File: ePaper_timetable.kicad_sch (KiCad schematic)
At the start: 44 parts, among them J1 26 pin FPC connector 0.5 mm p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, J2 Charging input - 5V, J3 Jumpers, J4 Jumpers, J5 Battery connector, Q1 NMOS, Q2 FS8205A, Q3 PMOS, SW1 SW_Push, SW2 SW_Push, SW3 SW_Push, U1 TP4056, U2 DW01A

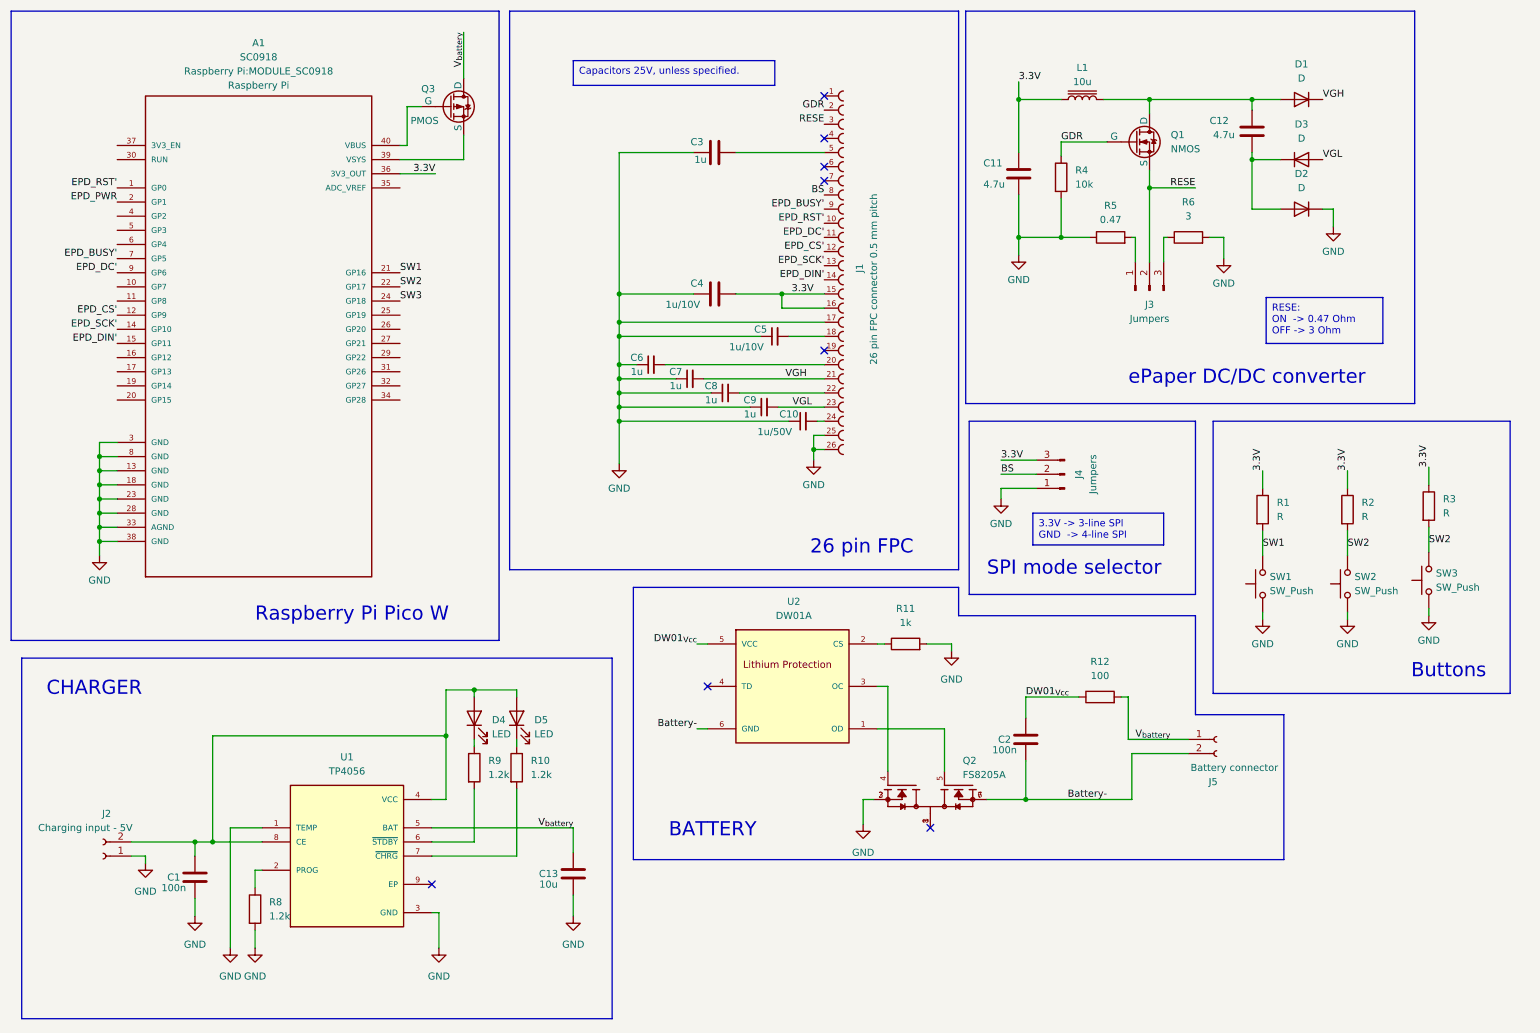
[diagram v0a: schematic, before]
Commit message: reference board
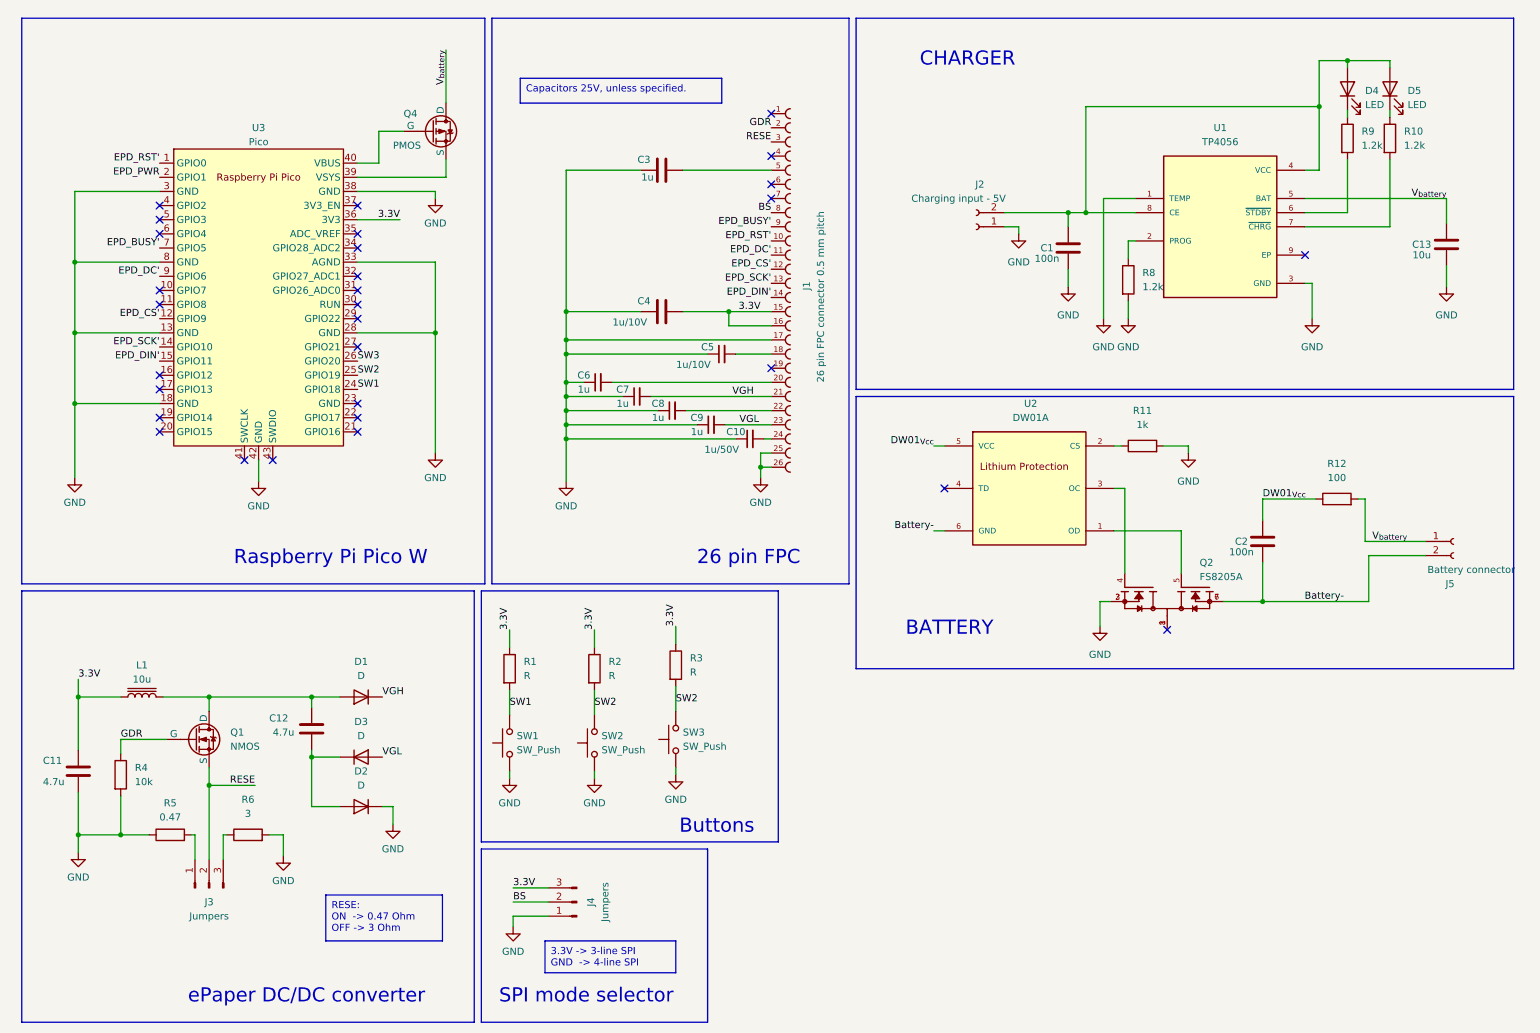
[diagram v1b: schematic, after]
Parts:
- removed A1: SC0918, Raspberry Pi:MODULE_SC0918, symbol Raspberry_Pi_Pico_W_SC0918:SC0918
- removed Q3: PMOS, symbol Simulation_SPICE:PMOS
- added Q4: PMOS, symbol Simulation_SPICE:PMOS
- added U3: Pico, RPi_Pico:RPi_Pico_SMD_TH, symbol MCU_RaspberryPi_and_Boards:Pico
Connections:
- net 3.3V: now also U3.36 (3V3)
- net EPD_BUSY': now also U3.7 (GPIO5)
- net EPD_CS': now also U3.12 (GPIO9)
- net EPD_DC': now also U3.9 (GPIO6)
- net EPD_DIN': now also U3.15 (GPIO11)
- net EPD_PWR: now also U3.2 (GPIO1)
- net EPD_RST': now also U3.1 (GPIO0)
- net EPD_SCK': now also U3.14 (GPIO10)
- net GND: now also U3.13 (GND), U3.18 (GND), U3.28 (GND), U3.3 (GND), U3.33 (AGND), U3.38 (GND), U3.42 (GND), U3.8 (GND)
- net SW1: now also U3.24 (GPIO18)
- net SW2: now also U3.25 (GPIO19)
- net SW3: now also U3.26 (GPIO20)
- net V_{battery}: now also Q4.1 (D)
- new net: Q4.2 (G), U3.40 (VBUS)
- new net: Q4.3 (S), U3.39 (VSYS)
- no-connect marks 8 -> 30
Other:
- moved on the sheet: C1, C10, C11, C12, C13, C2, C3, C4, C5, C6, C7, C8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
